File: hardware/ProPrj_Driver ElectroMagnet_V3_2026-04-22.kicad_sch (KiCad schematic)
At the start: 26 parts, among them CN4 BM06B-SRSS-TBT(LF)(SN), U4 DRV8210DSGR, U5 DRV8210DSGR, U6 DRV8210DSGR

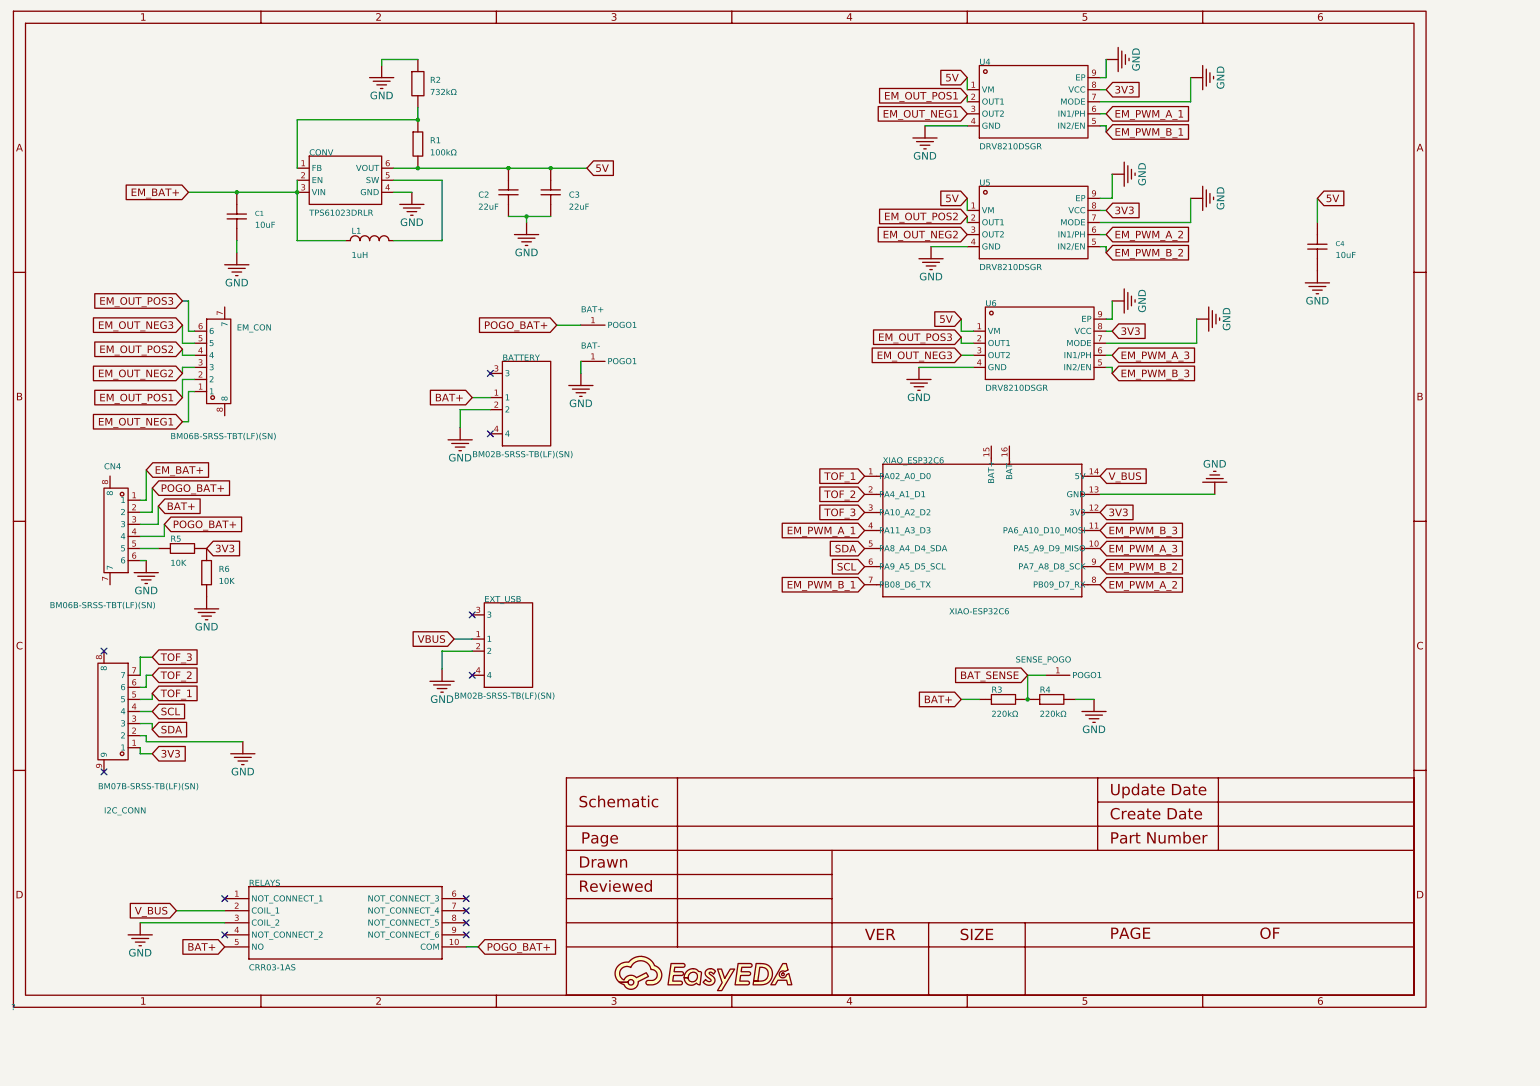
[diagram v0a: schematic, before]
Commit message: Modified readme
Co-authored-by: Copilot <copilot@github.com>
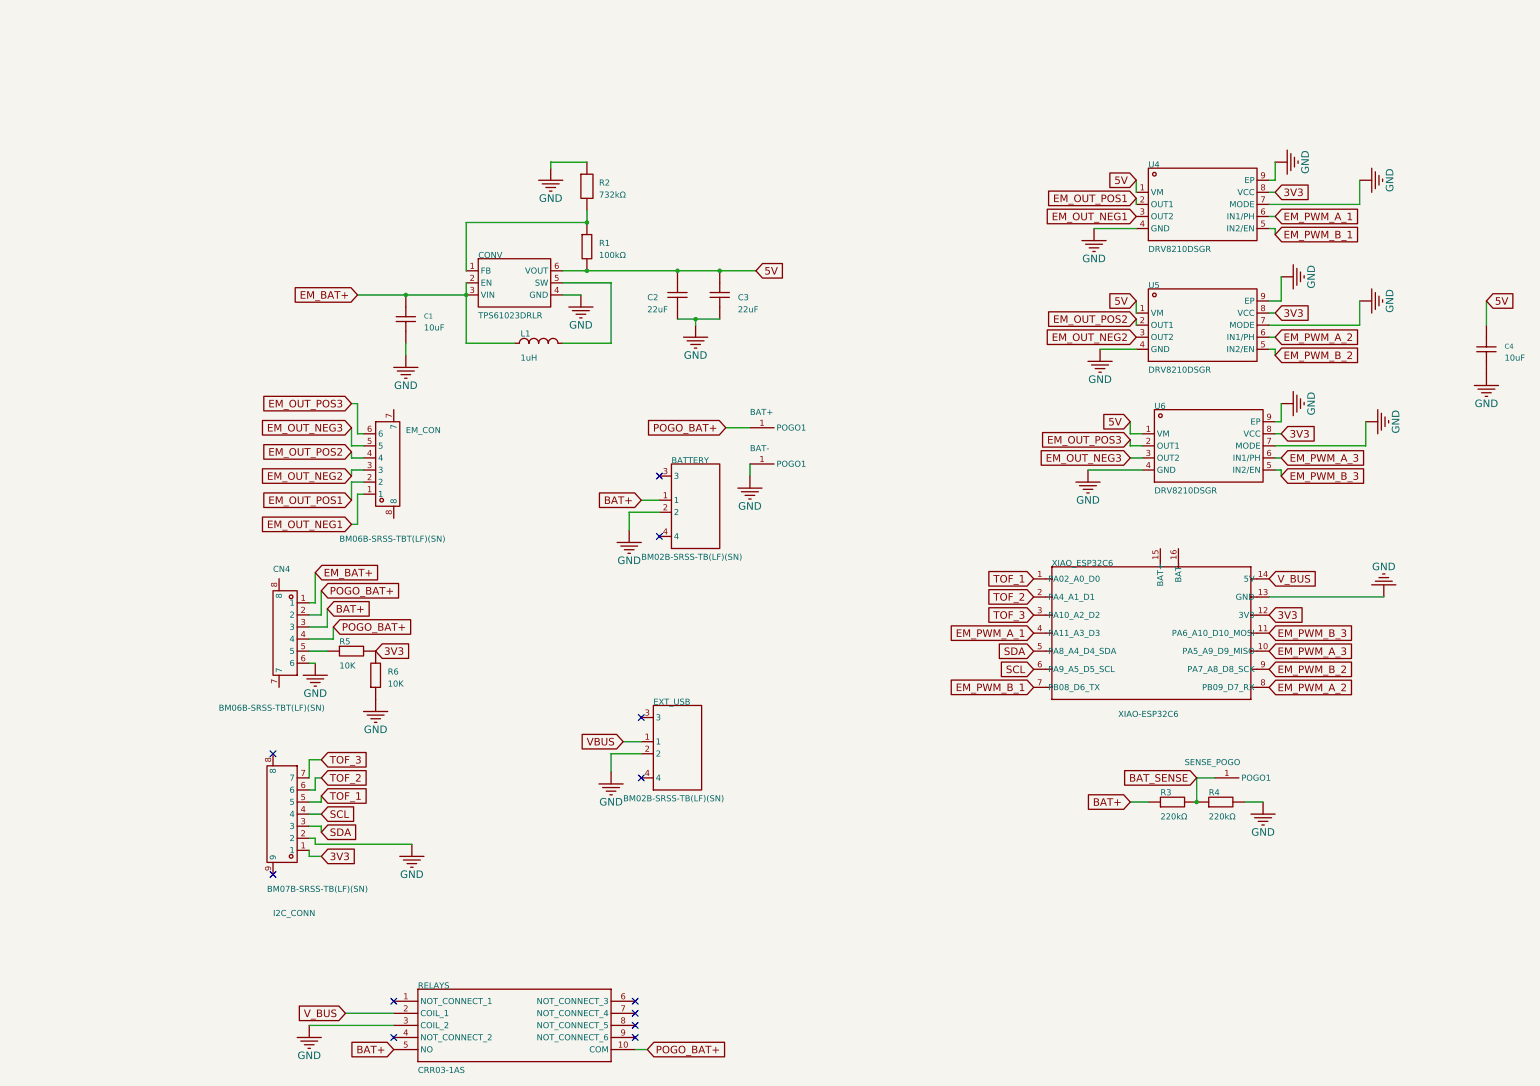
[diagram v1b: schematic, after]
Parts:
- removed ?: (no value), ProPrj_Dri-easyedapro:, symbol ProPrj_Dri-easyedapro:Sheet-Symbol_A4
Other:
- moved on the sheet: BAT+, BAT-, BATTERY, C1, C2, C3, C4, CN4, CONV, EM_CON, EXT_USB, I2C_CONN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
